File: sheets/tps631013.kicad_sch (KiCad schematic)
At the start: 6 parts, among them U5 TPS631011

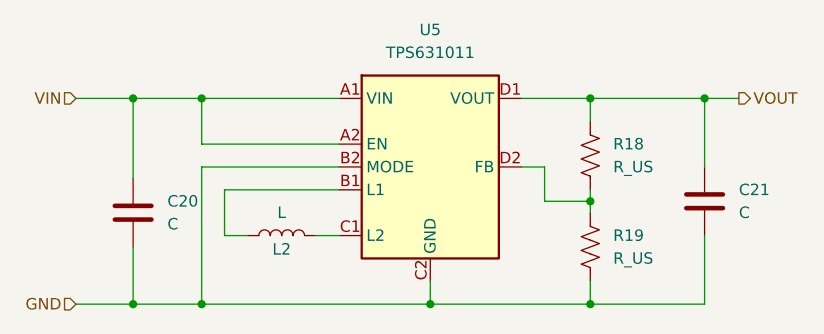
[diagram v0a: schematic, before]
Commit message: Some changes for powerups
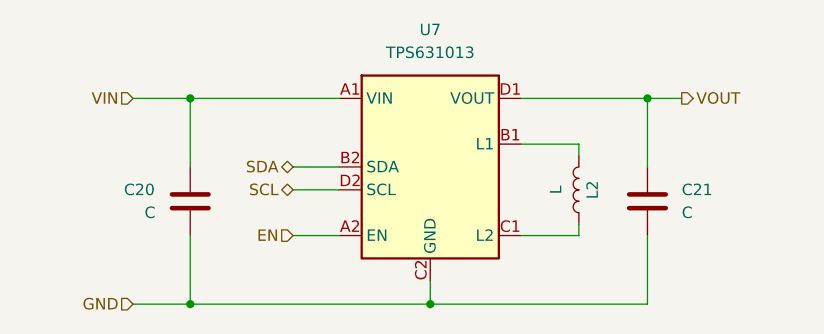
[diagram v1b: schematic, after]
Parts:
- removed R18, R19: R_US, symbol Device:R_US
- removed U5: TPS631011, symbol PowerFeather_KiCAD_Lib:TPS631011
- added U7: TPS631013, symbol PowerFeather_KiCAD_Lib:TPS631013
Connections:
- net GND: now also U7.C2 (GND)
- net VIN: now also U7.A1 (VIN)
- net VOUT: now also U7.D1 (VOUT)
- net at L2.1: now also U7.C1 (L2)
- net at L2.2: now also U7.B1 (L1)
- new net EN: U7.A2 (EN)
- new net SCL: U7.D2 (SCL)
- new net SDA: U7.B2 (SDA)
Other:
- moved on the sheet: C20, C21, L2
